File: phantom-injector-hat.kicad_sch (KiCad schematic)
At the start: 40 parts, among them J1 Conn_02x20_Odd_Even, J2 Conn_02x03_Top_Bottom, J3 Conn_01x03, J4 Conn_01x03, SW1 SW_SPST, U1 LT8362EMSE-PBF

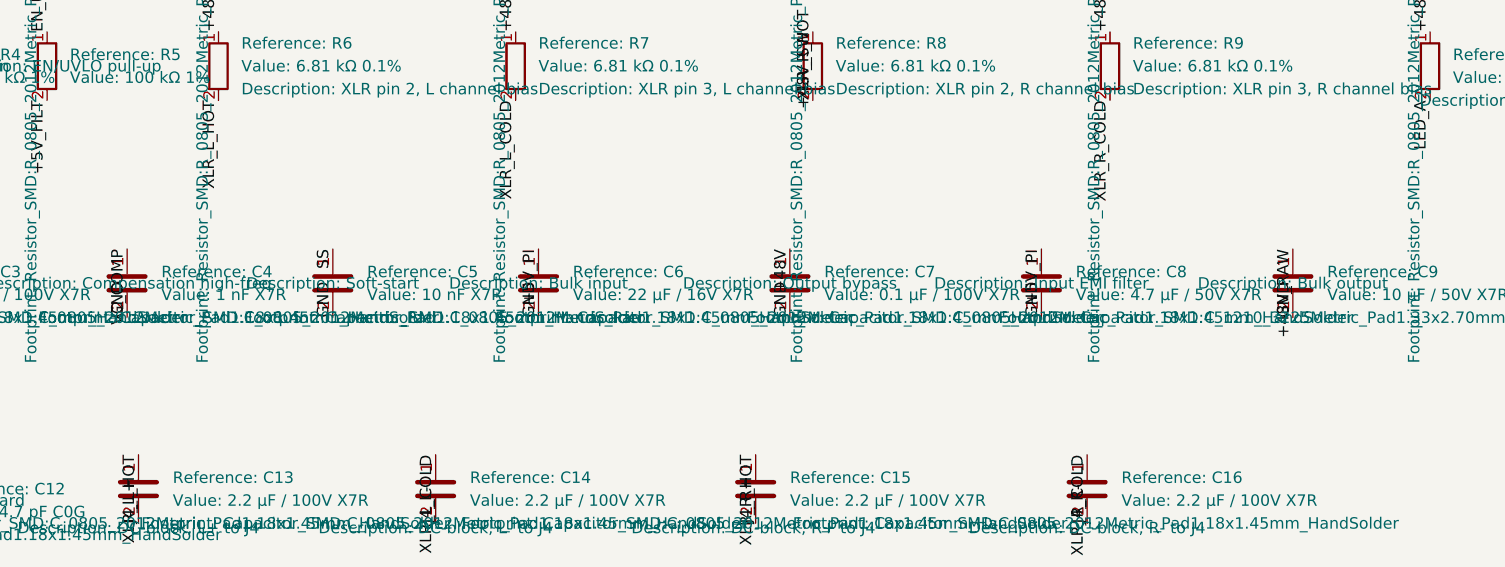
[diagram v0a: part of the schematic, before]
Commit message: WIP
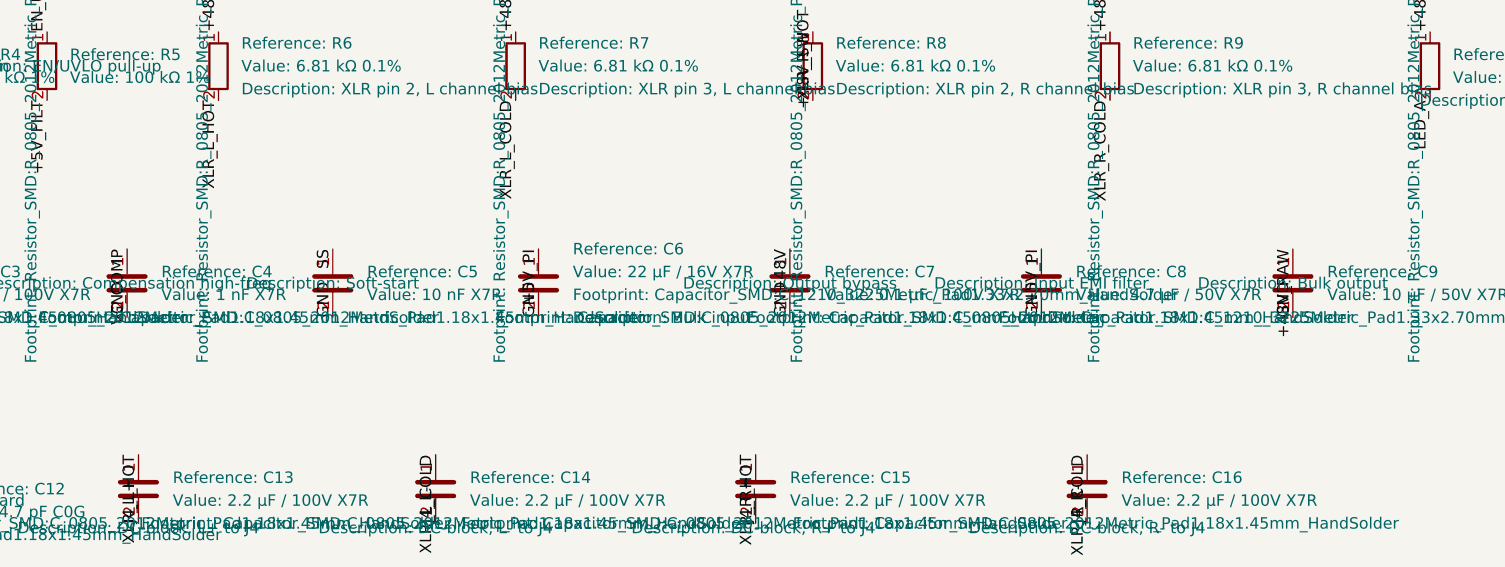
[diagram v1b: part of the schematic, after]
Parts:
- C6: footprint Capacitor_SMD:C_0805_2012Metric_Pad1.18x1.45mm_HandSolder -> Capacitor_SMD:C_1210_3225Metric_Pad1.33x2.70mm_HandSolder
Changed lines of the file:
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@@
 		(fields_autoplaced yes)
 		(property "Reference" "C6"
+			(at 166.37 78.7399 0)
+			(show_name yes)
+			(do_not_autoplace no)
+			(effects
+				(font
+					(size 1.27 1.27)
+				)
+				(justify left)
+			)
+		)
+		(property "Value" "22 µF / 16V X7R"
 			(at 166.37 81.2799 0)
 			(show_name yes)
@@
 			)
 		)
-		(property "Value" "22 µF / 16V X7R"
+		(property "Footprint" "Capacitor_SMD:C_1210_3225Metric_Pad1.33x2.70mm_HandSolder"
 			(at 166.37 83.8199 0)
 			(show_name yes)
@@
 				)
 				(justify left)
-			)
-		)
-		(property "Footprint" "Capacitor_SMD:C_0805_2012Metric_Pad1.18x1.45mm_HandSolder"
-			(at 163.5252 86.36 0)
-			(show_name yes)
-			(do_not_autoplace no)
-			(effects
-				(font
-					(size 1.27 1.27)
-				)
 			)
 		)
@@
 		)
 		(property "Description" "Bulk input"
-			(at 162.56 82.55 0)
+			(at 166.37 86.3599 0)
 			(show_name yes)
 			(do_not_autoplace no)
@@
 					(size 1.27 1.27)
 				)
+				(justify left)
 			)
 		)
